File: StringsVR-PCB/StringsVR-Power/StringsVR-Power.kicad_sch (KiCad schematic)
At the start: 19 parts, among them J1 MPU6050, J2 Conn_02x20_Odd_Even, SW1 ON/OFF

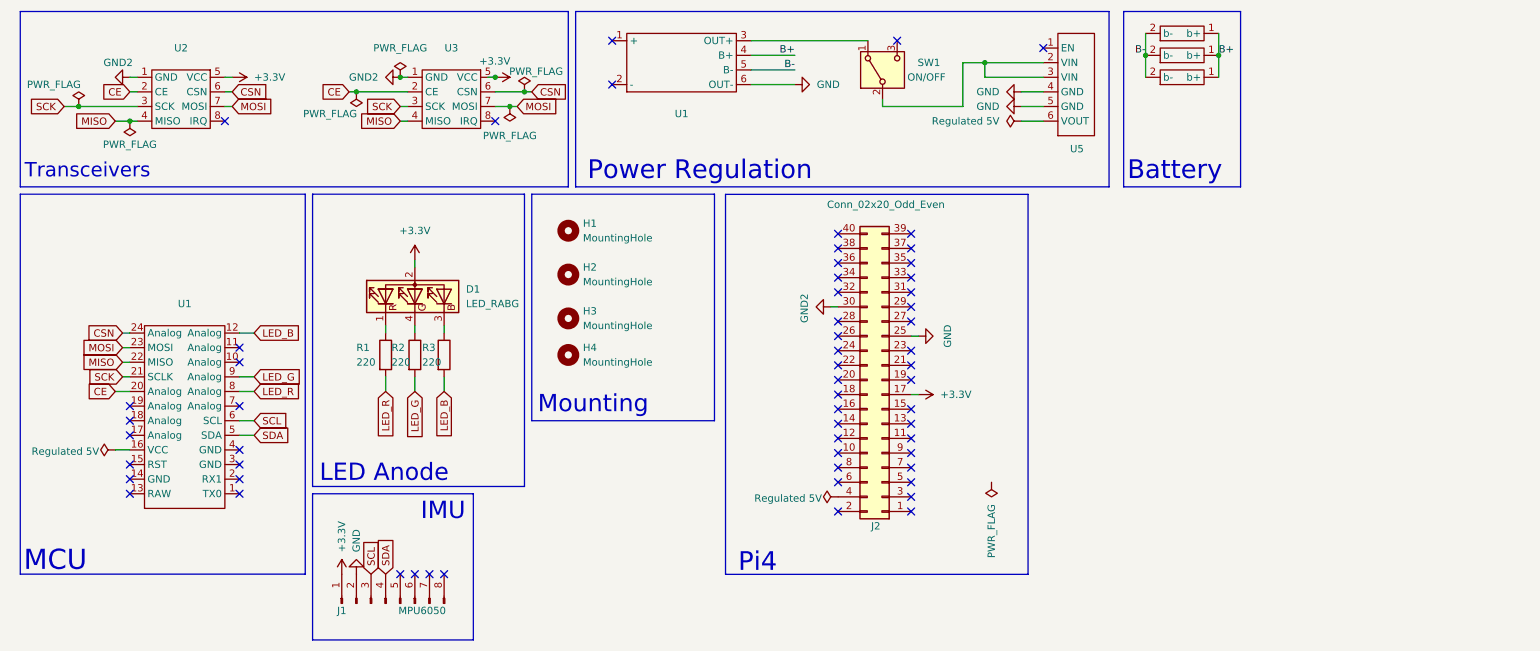
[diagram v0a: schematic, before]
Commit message: moved my changes to separate folder
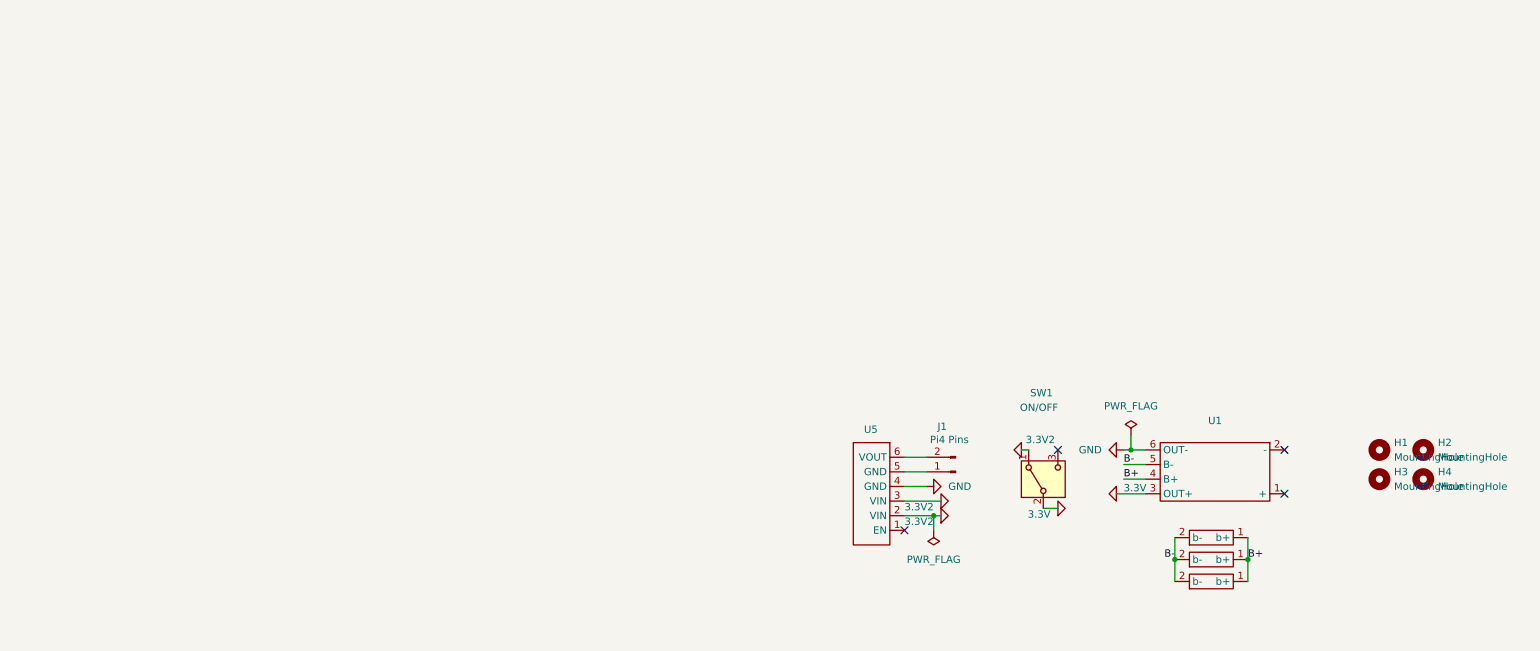
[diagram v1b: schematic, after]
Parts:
- removed D1: LED_RABG, LED_THT:LED_D5.0mm-4_RGB, symbol Device:LED_RABG
- removed J1: MPU6050, Arduino:MPU6050, symbol Connector:Conn_01x08_Pin
- removed J2: Conn_02x20_Odd_Even, Arduino:Pin_Header_Straight_2x20_Pitch2.54mm, symbol Connector_Generic:Conn_02x20_Odd_Even
- removed R1, R2, R3: 220, Resistor_SMD:R_0603_1608Metric, symbol Device:R
- removed U1: ~, Arduino:Pro Micro, symbol Arduino:Pro_Micro
- removed U2, U3: ~, Arduino:nRF24L01, symbol Arduino:nRF24L01
- added J1: Pi4 Pins, Connector_PinHeader_2.54mm:PinHeader_1x02_P2.54mm_Vertical, symbol Connector:Conn_01x02_Pin
- H1, H2, H3, H4: footprint MountingHole:MountingHole_2.7mm -> MountingHole:MountingHole_2.5mm
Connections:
- net GND: no longer U5.5 (GND)
- net 3.3V2: now reaches U5.2 (VIN), U5.3 (VIN)
- net 3.3V2: now also SW1.1 (A); no longer SW1.2 (B)
- net at U5.6 (VOUT): now also J1.2 (Pin_2)
- net 3.3V: now reaches U1.3 (OUT+)
- net 3.3V: now also SW1.2 (B); no longer SW1.1 (A)
- new net: J1.1 (Pin_1), U5.5 (GND)
- no-connect marks 59 -> 4
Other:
- note removed: "Battery"
- note removed: "IMU"
- note removed: "LED Anode"
- note removed: "MCU"
- note removed: "Mounting"
- note removed: "Pi4"
- note removed: "Power Regulation"
- note removed: "Transceivers"
- moved on the sheet: SW1, U1, U5

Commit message: new integrated board
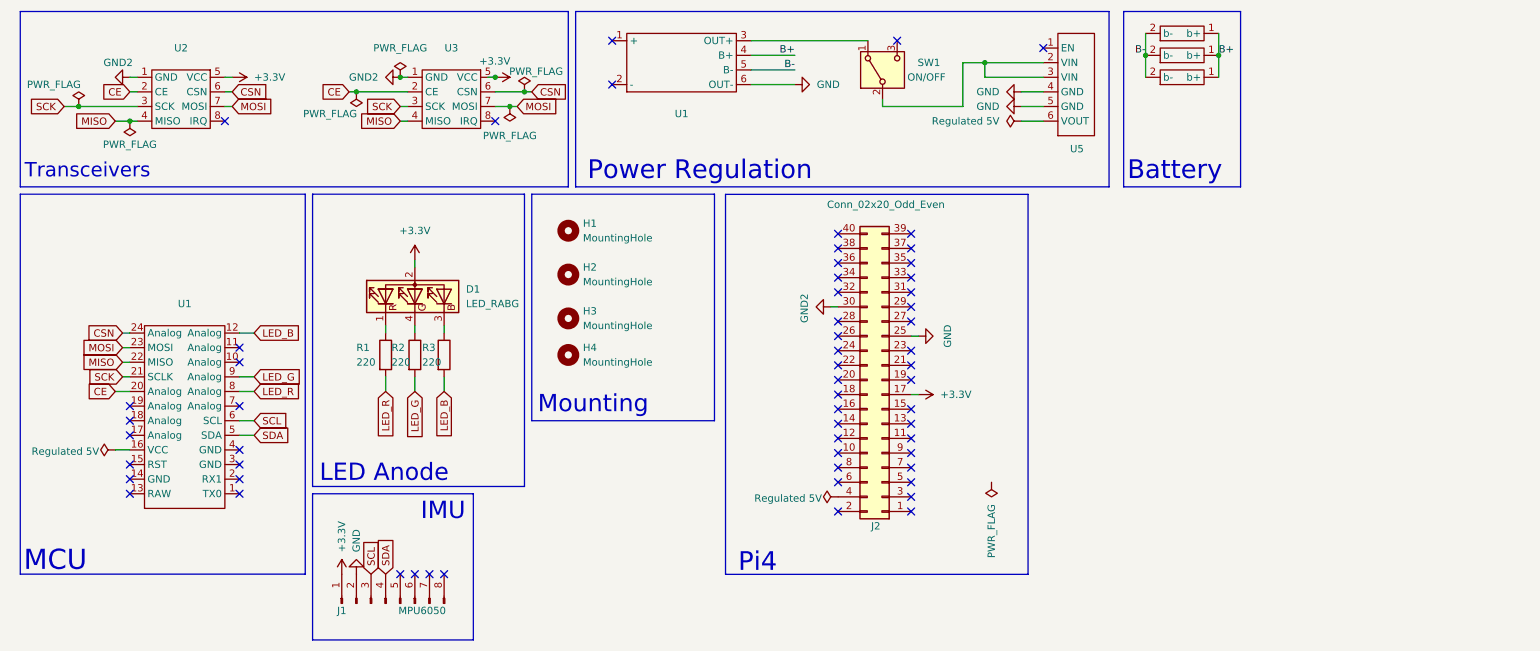
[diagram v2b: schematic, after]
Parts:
- removed J1: Pi4 Pins, Connector_PinHeader_2.54mm:PinHeader_1x02_P2.54mm_Vertical, symbol Connector:Conn_01x02_Pin
- added D1: LED_RABG, LED_THT:LED_D5.0mm-4_RGB, symbol Device:LED_RABG
- added J1: MPU6050, Arduino:MPU6050, symbol Connector:Conn_01x08_Pin
- added J2: Conn_02x20_Odd_Even, Arduino:Pin_Header_Straight_2x20_Pitch2.54mm, symbol Connector_Generic:Conn_02x20_Odd_Even
- added R1, R2, R3: 220, Resistor_SMD:R_0603_1608Metric, symbol Device:R
- added U1: ~, Arduino:Pro Micro, symbol Arduino:Pro_Micro
- added U2, U3: ~, Arduino:nRF24L01, symbol Arduino:nRF24L01
- H1, H2, H3, H4: footprint MountingHole:MountingHole_2.5mm -> MountingHole:MountingHole_2.7mm
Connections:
- net GND: now also U5.5 (GND), J1.2 (Pin_2), J2.25 (Pin_25)
- net 3.3V: no longer names the net of SW1.2 (B)
- net 3.3V: now also U5.2 (VIN), U5.3 (VIN); no longer U1.3 (OUT+)
- removed net 3.3V2: SW1.1 (A), U5.2 (VIN), U5.3 (VIN)
- new net: D1.3 (BK), R3.1
- new net: D1.1 (RK), R1.1
- new net: D1.4 (GK), R2.1
- new net: SW1.1 (A), U1.3 (OUT+)
- new net +3.3V: D1.2 (A), J1.1 (Pin_1), J2.17 (Pin_17), U2.5 (VCC), U3.5 (VCC)
- new net CE: U1.20 (Analog), U2.2 (CE), U3.2 (CE)
- new net CSN: U1.24 (Analog), U2.6 (CSN), U3.6 (CSN)
- new net GND2: J2.30 (Pin_30), U2.1 (GND), U3.1 (GND)
- new net LED_B: R3.2, U1.12 (Analog)
- new net LED_G: R2.2, U1.9 (Analog)
- new net LED_R: R1.2, U1.8 (Analog)
- new net MISO: U1.22 (MISO), U2.4 (MISO), U3.4 (MISO)
- new net MOSI: U1.23 (MOSI), U2.7 (MOSI), U3.7 (MOSI)
- new net SCK: U1.21 (SCLK), U2.3 (SCK), U3.3 (SCK)
- new net SCL: J1.3 (Pin_3), U1.6 (SCL)
- new net SDA: J1.4 (Pin_4), U1.5 (SDA)
- no-connect marks 4 -> 59
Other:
- note added: "Battery"
- note added: "IMU"
- note added: "LED Anode"
- note added: "MCU"
- note added: "Mounting"
- note added: "Pi4"
- note added: "Power Regulation"
- note added: "Transceivers"
- moved on the sheet: SW1, U1, U5
